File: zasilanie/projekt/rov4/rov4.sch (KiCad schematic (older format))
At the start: 70 parts, among them IC1 UWE-12_10-Q12PB-C, J1 Reed switch, J10 Switch, J11 BatteryPower, J12 RC_D_12V, J13 Xavier, J14 Kamera 1, J15 Kamera 2, J16 Extra, J17 Extra, J18 Hydrofony, J19 Extra, J2 Battery digital, J20 Extra, J21 Extra, J22 RC_D_15V, J3 Manip_SterSil2, J37 STM32, J4 Manip_SterSil1, J47 Enko_inkrementalny, J48 Torpedy, hall, laser, J49 Enko_absolutny_1, J5 Extra, J50 Enko_absolutny_2, J6 Extra, J7 RC_D_5V, J8 RPi, J9 Router, Q1 IPT004N03L, Q2 IPT004N03L, Q3 BC847A, Q4 BC847A, Q5 BC847A, U1 lm2596

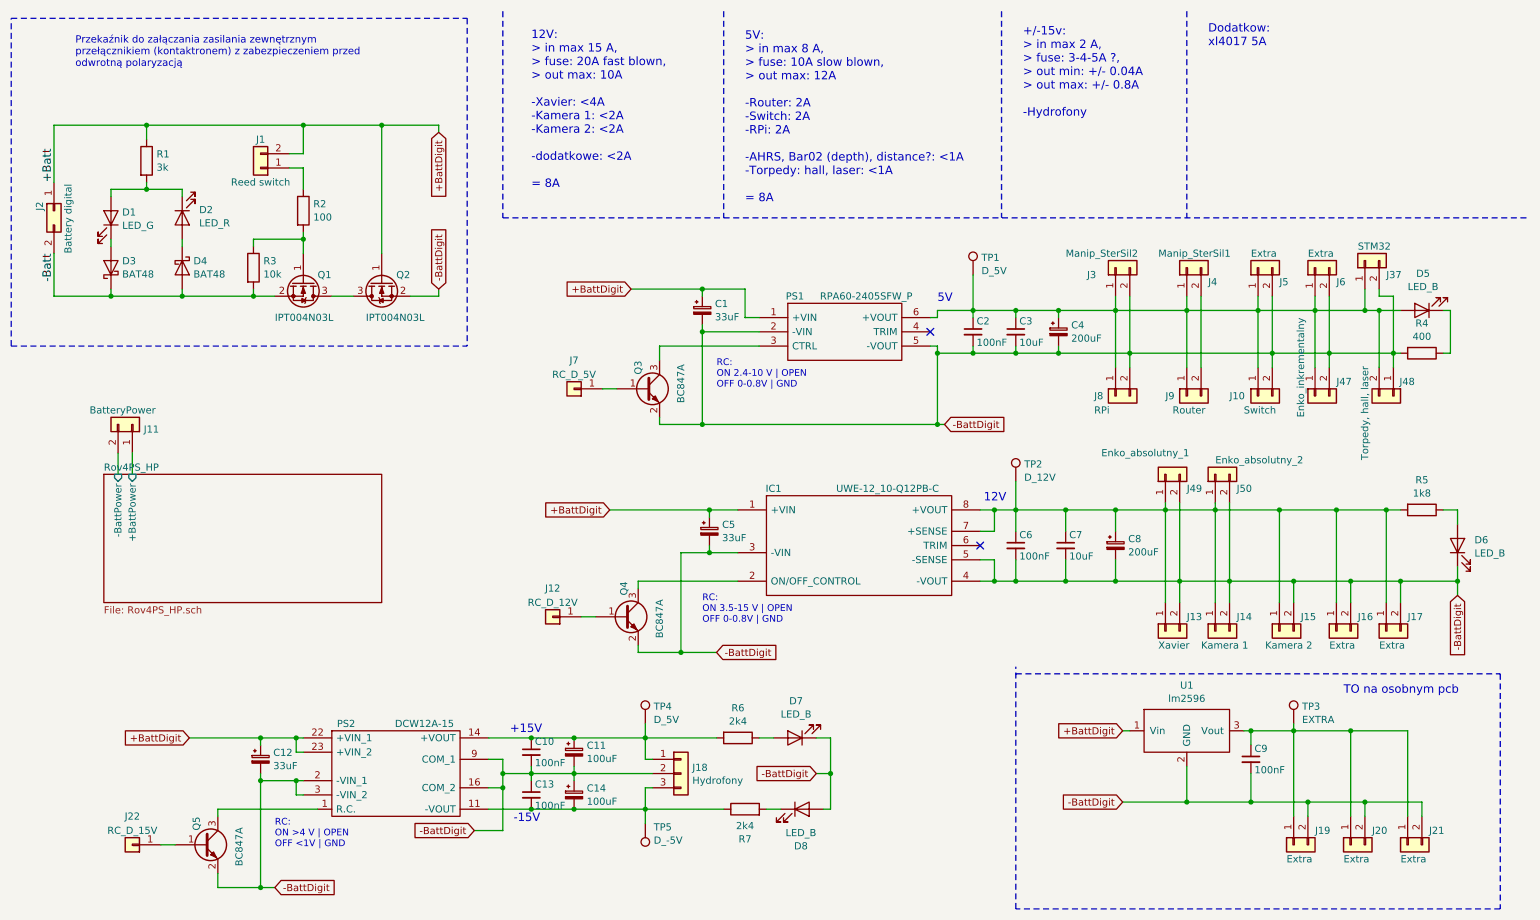
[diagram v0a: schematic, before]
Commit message: Reorganizacja struktury projektu
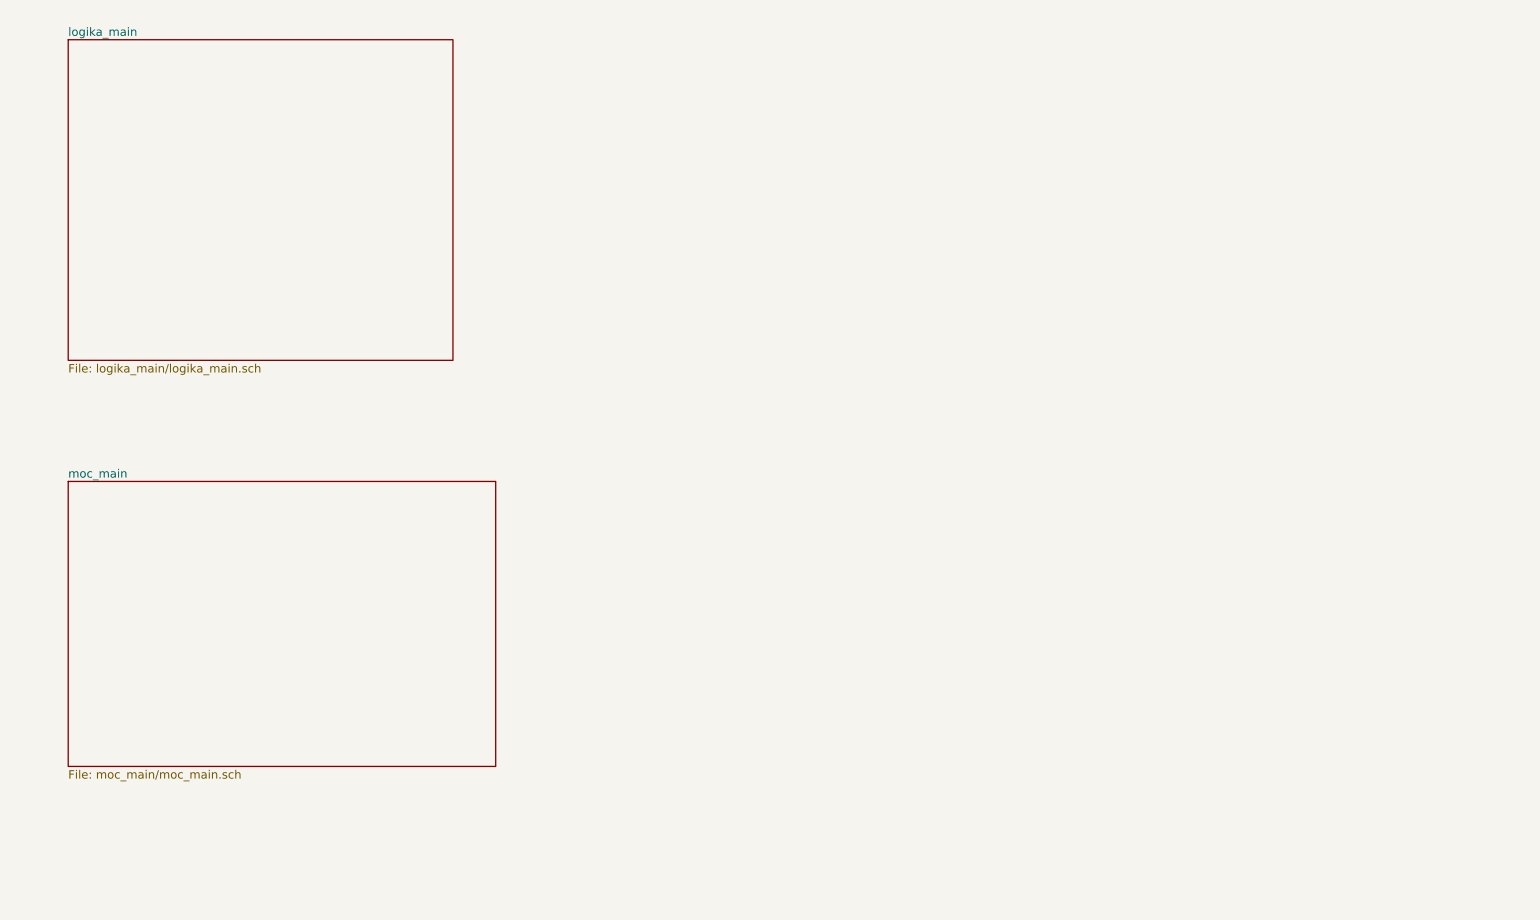
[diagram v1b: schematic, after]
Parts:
- removed C1, C12, C5: 33uF, Capacitor_SMD:CP_Elec_6.3x5.4, symbol Device:CP_Small
- removed C10, C13, C2, C6, C9: 100nF, Capacitor_SMD:C_0805_2012Metric, symbol Device:C_Small
- removed C11, C14: 100uF, Capacitor_SMD:CP_Elec_6.3x7.7, symbol Device:CP_Small
- removed C3, C7: 10uF, Capacitor_SMD:C_0805_2012Metric, symbol Device:C_Small
- removed C4, C8: 200uF, Capacitor_SMD:CP_Elec_8x10, symbol Device:CP_Small
- removed D1: LED_G, LED_SMD:LED_0805_2012Metric, symbol Device:LED
- removed D2: LED_R, LED_SMD:LED_0805_2012Metric, symbol Device:LED
- removed D3, D4: BAT48, Diode_SMD:D_MiniMELF, symbol Device:D_Schottky
- removed D5, D6, D7, D8: LED_B, LED_SMD:LED_0805_2012Metric, symbol Device:LED
- removed IC1: UWE-12_10-Q12PB-C, UWE-12_10-Q12P-C:UWE-12_10-Q12P-C, symbol UWE-12_10-Q12P-C:UWE-12_10-Q12PB-C
- removed J1: Reed switch, Connector_PinHeader_2.54mm:PinHeader_1x02_P2.54mm_Vertical, symbol Connector_Generic:Conn_01x02
- removed J10: Switch, Connector_PinHeader_2.54mm:PinHeader_1x02_P2.54mm_Vertical, symbol Connector_Generic:Conn_01x02
- removed J11: BatteryPower, Connector_PinHeader_2.54mm:PinHeader_1x02_P2.54mm_Vertical, symbol Connector_Generic:Conn_01x02
- removed J12: RC_D_12V, Connector_PinHeader_2.54mm:PinHeader_1x01_P2.54mm_Vertical, symbol Connector_Generic:Conn_01x01
- removed J13: Xavier, Connector_PinHeader_2.54mm:PinHeader_1x02_P2.54mm_Vertical, symbol Connector_Generic:Conn_01x02
- removed J14: Kamera 1, Connector_PinHeader_2.54mm:PinHeader_1x02_P2.54mm_Vertical, symbol Connector_Generic:Conn_01x02
- removed J15: Kamera 2, Connector_PinHeader_2.54mm:PinHeader_1x02_P2.54mm_Vertical, symbol Connector_Generic:Conn_01x02
- removed J16, J17, J21, J5, J6: Extra, Connector_PinHeader_2.54mm:PinHeader_1x02_P2.54mm_Vertical, symbol Connector_Generic:Conn_01x02
- removed J18: Hydrofony, Connector_PinHeader_2.54mm:PinHeader_1x03_P2.54mm_Vertical, symbol Connector_Generic:Conn_01x03
- removed J19: Extra, Connector_Molex:Molex_SPOX_5267-02A_1x02_P2.50mm_Vertical, symbol Connector_Generic:Conn_01x02
- removed J2: Battery digital, Connector_PinSocket_2.54mm:PinSocket_2x01_P2.54mm_Vertical, symbol Connector_Generic:Conn_02x01
- removed J20: Extra, Connector_Molex:Molex_Mini-Fit_Jr_5566-02A_2x01_P4.20mm_Vertical, symbol Connector_Generic:Conn_01x02
- removed J22: RC_D_15V, Connector_PinHeader_2.54mm:PinHeader_1x01_P2.54mm_Vertical, symbol Connector_Generic:Conn_01x01
- removed J3: Manip_SterSil2, Connector_PinHeader_2.54mm:PinHeader_1x02_P2.54mm_Vertical, symbol Connector_Generic:Conn_01x02
- removed J37: STM32, Connector_PinHeader_2.54mm:PinHeader_1x02_P2.54mm_Vertical, symbol Connector_Generic:Conn_01x02
- removed J4: Manip_SterSil1, Connector_PinHeader_2.54mm:PinHeader_1x02_P2.54mm_Vertical, symbol Connector_Generic:Conn_01x02
- removed J47: Enko_inkrementalny, Connector_PinHeader_2.54mm:PinHeader_1x02_P2.54mm_Vertical, symbol Connector_Generic:Conn_01x02
- removed J48: Torpedy, hall, laser, Connector_PinHeader_2.54mm:PinHeader_1x02_P2.54mm_Vertical, symbol Connector_Generic:Conn_01x02
- removed J49: Enko_absolutny_1, Connector_PinHeader_2.54mm:PinHeader_1x02_P2.54mm_Vertical, symbol Connector_Generic:Conn_01x02
- removed J50: Enko_absolutny_2, Connector_PinHeader_2.54mm:PinHeader_1x02_P2.54mm_Vertical, symbol Connector_Generic:Conn_01x02
- removed J7: RC_D_5V, Connector_PinHeader_2.54mm:PinHeader_1x01_P2.54mm_Vertical, symbol Connector_Generic:Conn_01x01
- removed J8: RPi, Connector_PinHeader_2.54mm:PinHeader_1x02_P2.54mm_Vertical, symbol Connector_Generic:Conn_01x02
- removed J9: Router, Connector_PinHeader_2.54mm:PinHeader_1x02_P2.54mm_Vertical, symbol Connector_Generic:Conn_01x02
- removed PS1: RPA60-2405SFW_P, RPA60-2405SFW_P:RPA60-2405SFW_P, symbol RPA60-2405SFW_P:RPA60-2405SFW_P
- removed PS2: DCW12A-15, DCW12A-15:DCW12A-15, symbol DCW12A-15:DCW12A-15
- removed Q1, Q2: IPT004N03L, Package_TO_SOT_SMD:Infineon_PG-HSOF-8-1, symbol Device:Q_NMOS_GSD
- removed Q3, Q4, Q5: BC847A, Package_TO_SOT_SMD:SOT-23, symbol Device:Q_NPN_BEC
- removed R1: 3k, Resistor_SMD:R_0805_2012Metric, symbol Device:R
- removed R2: 100, Resistor_SMD:R_0805_2012Metric, symbol Device:R
- removed R3: 10k, Resistor_SMD:R_0805_2012Metric, symbol Device:R
- removed R4: 400, Resistor_SMD:R_0805_2012Metric, symbol Device:R
- removed R5: 1k8, Resistor_SMD:R_0805_2012Metric, symbol Device:R
- removed R6, R7: 2k4, Resistor_SMD:R_0805_2012Metric, symbol Device:R
- removed TP1, TP4: D_5V, Connector_PinHeader_2.54mm:PinHeader_1x01_P2.54mm_Vertical, symbol Connector:TestPoint
- removed TP2: D_12V, Connector_PinHeader_2.54mm:PinHeader_1x01_P2.54mm_Vertical, symbol Connector:TestPoint
- removed TP3: EXTRA, Connector_PinHeader_2.54mm:PinHeader_1x01_P2.54mm_Vertical, symbol Connector:TestPoint
- removed TP5: D_-5V, Connector_PinHeader_2.54mm:PinHeader_1x01_P2.54mm_Vertical, symbol Connector:TestPoint
- removed U1: lm2596, lm2596:lm2596-44_8mm_x_23mm, symbol lm2596:lm2596
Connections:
- no-connect marks 2 -> 0
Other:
- note removed: "+/-15v:\n> in max 2 A,\n> fuse: 3-4-5A ?,\n> out min: +/- 0.04A\n> out max: +/- 0.8A\n\n-Hydrofony\n"
- note removed: "+15V"
- note removed: "-15V"
- note removed: "12V"
- note removed: "12V:\n> in max 15 A,\n> fuse: 20A fast blown,\n> out max: 10A\n\n-Xavier: <4A\n-Kamera 1: <2A\n-Kamera 2: <2A\n\n-dodatkowe: <2A\n\n= 8A\n"
- note removed: "5V"
- note removed: "5V:\n> in max 8 A,\n> fuse: 10A slow blown,\n> out max: 12A\n\n-Router: 2A\n-Switch: 2A\n-RPi: 2A\n\n-AHRS, Bar02 (depth), distance?: <1A\n-Torpedy: hall, laser: <1A\n\n= 8A\n"
- note removed: "Dodatkow:\nxl4017 5A\n\n"
- note removed: "Przekaźnik do załączania zasilania zewnętrznym \nprzełącznikiem (kontaktronem) z zabezpieczeniem przed \nodwrotną polaryzacją"
- note removed: "RC:\nON 2.4-10 V | OPEN\nOFF 0-0.8V | GND"
- note removed: "RC:\nON 3.5-15 V | OPEN\nOFF 0-0.8V | GND"
- note removed: "RC:\nON >4 V | OPEN\nOFF <1V | GND"
- note removed: "TO na osobnym pcb"
